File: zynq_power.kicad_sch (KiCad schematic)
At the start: 1 part, among them U2 XC7Z020-2CLG400I

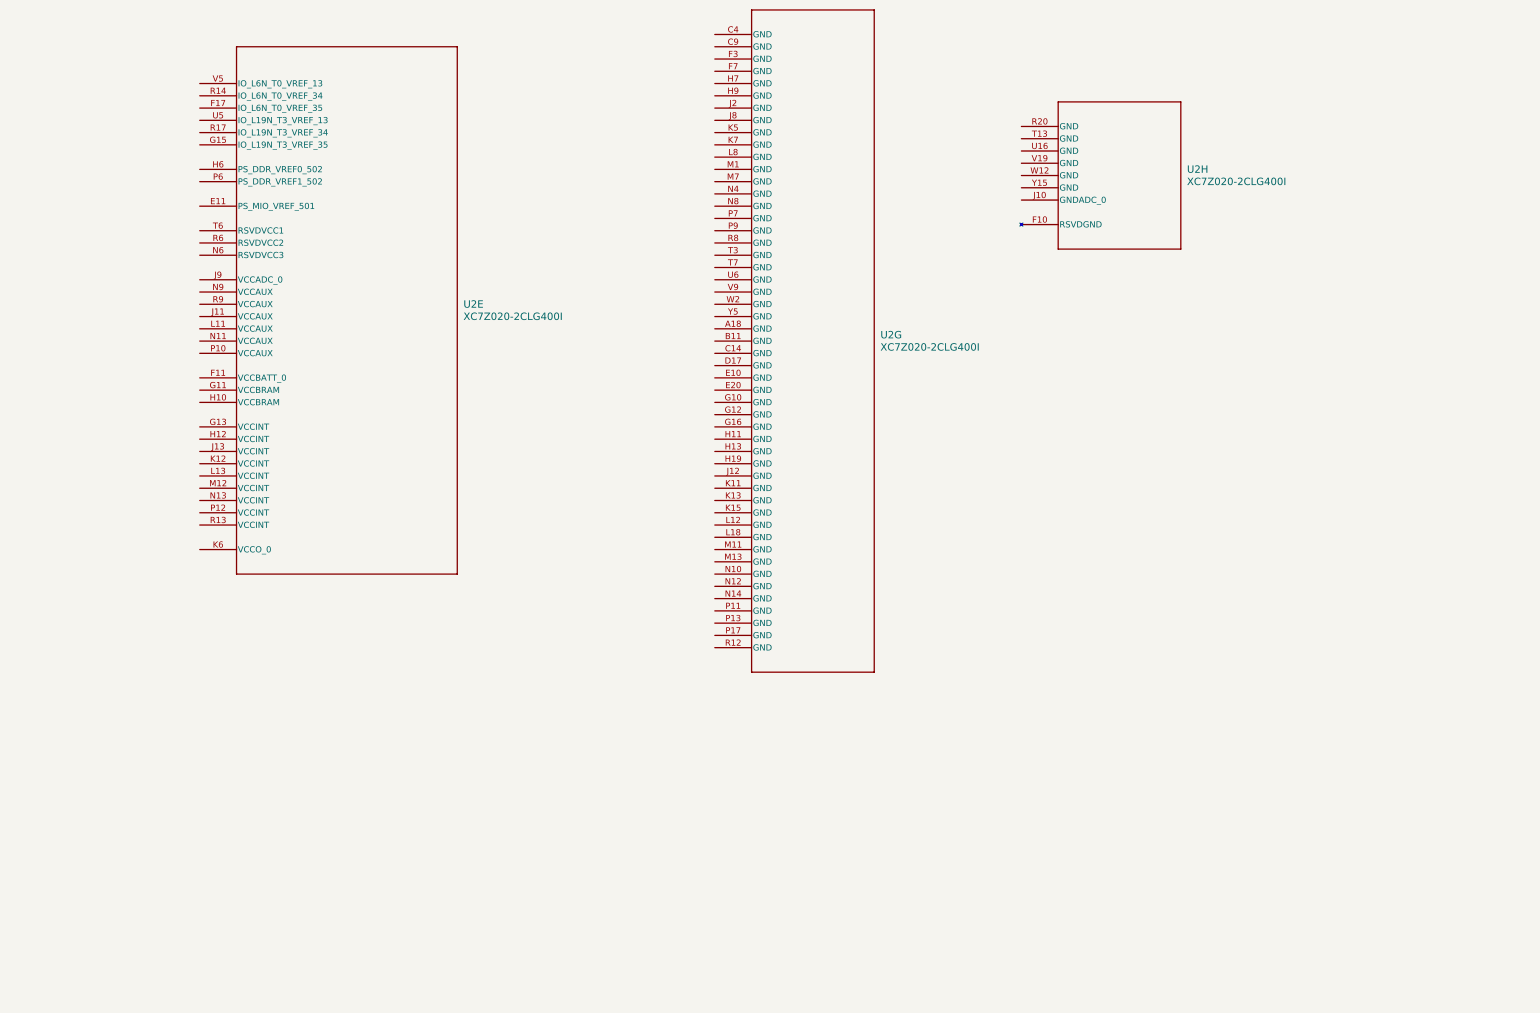
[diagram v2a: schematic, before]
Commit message: sch-updated
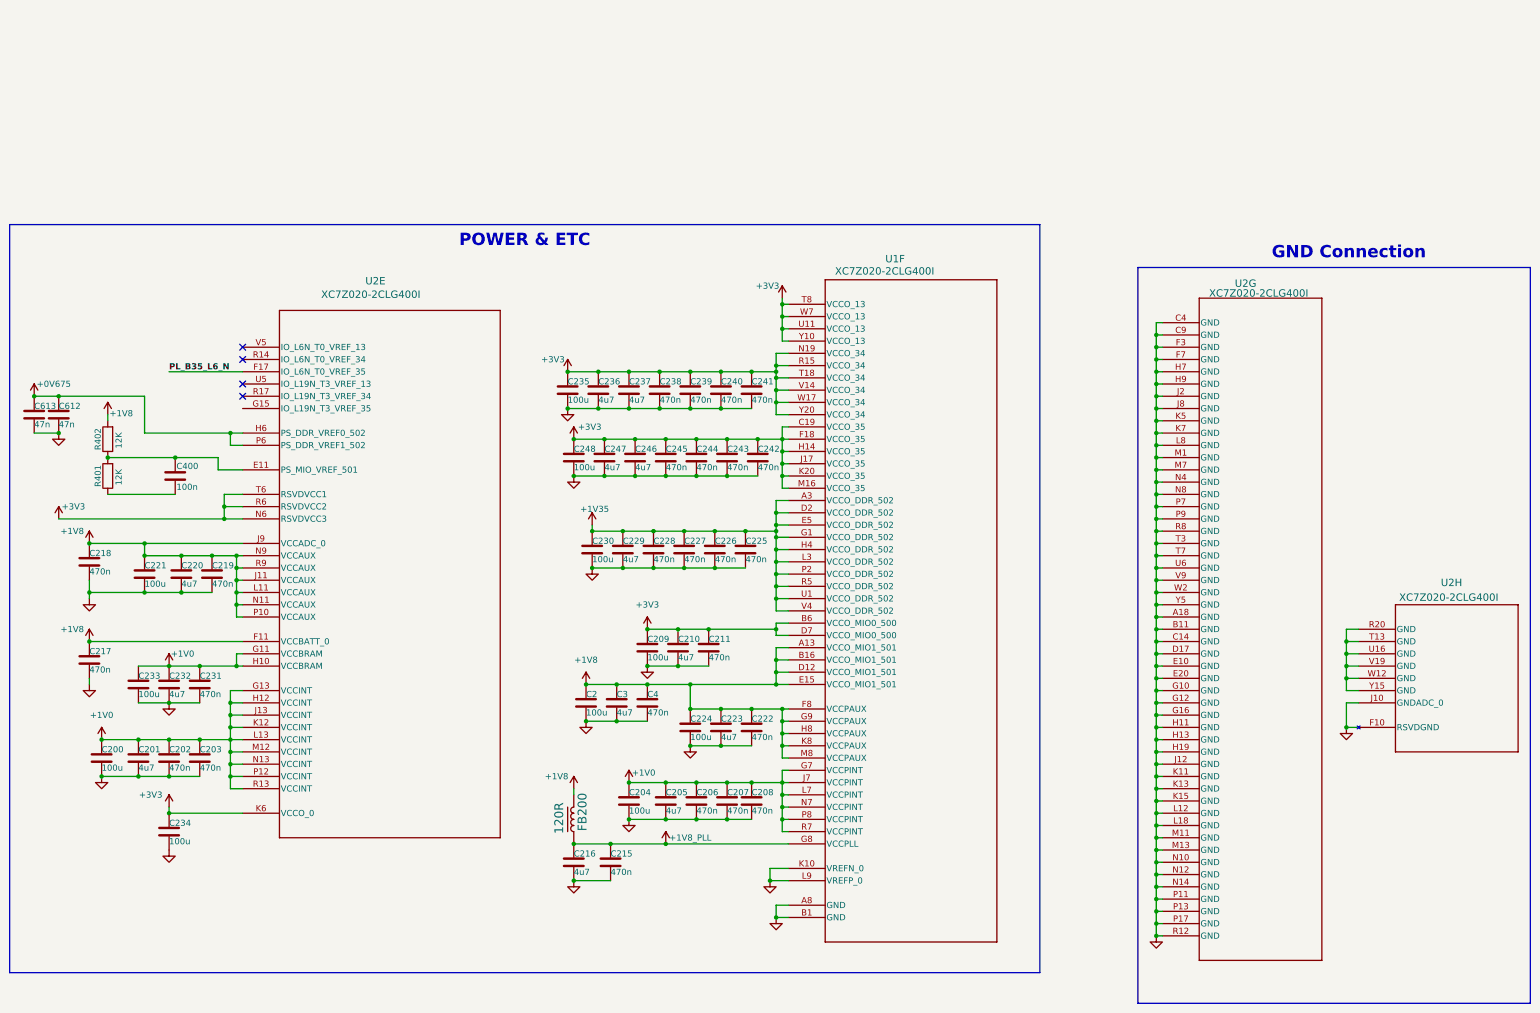
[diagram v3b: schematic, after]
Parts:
- added C2, C200, C204, C209, C221, C224, C230, C233, C234, C235, C248: 100u, Capacitor_SMD:C_1206_3216Metric, symbol Device:C
- added C201, C205, C210, C216, C220, C223, C229, C232, C236, C237, C246, C247, C3: 4u7, Capacitor_SMD:C_0402_1005Metric, symbol Device:C
- added C202, C203, C206, C207, C208, C211, C215, C217, C218, C219, C222, C225, C226, C227, C228, C231, C238, C239, C240, C241, C242, C243, C244, C245, C4: 470n, Capacitor_SMD:C_0402_1005Metric, symbol Device:C
- added C400: 100n, Capacitor_SMD:C_0402_1005Metric, symbol Device:C
- added C612, C613: 47n, Capacitor_SMD:C_0402_1005Metric, symbol Device:C
- added FB200: 120R, FB_0402, symbol Schematic-Lib-PhilsLab:FB_0402
- added R401, R402: 12K, Resistor_SMD:R_0402_1005Metric, symbol Device:R
- added U1: XC7Z020-2CLG400I, Package_BGA:Xilinx_CLG400, symbol 2024-11-30_12-42-37:XC7Z020-2CLG400I
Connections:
- net GND: now reaches U2.F10 (RSVDGND)
- net GND: now also U2.A18 (GND), U2.B11 (GND), U2.C14 (GND), U2.C4 (GND), U2.C9 (GND), U2.D17 (GND), U2.E10 (GND), U2.E20 (GND), U2.F3 (GND), U2.F7 (GND), U2.G10 (GND), U2.G12 (GND), U2.G16 (GND), U2.H11 (GND), U2.H13 (GND), U2.H19 (GND), U2.H7 (GND), U2.H9 (GND), U2.J10 (GNDADC_0), U2.J12 (GND), U2.J2 (GND), U2.J8 (GND), U2.K11 (GND), U2.K13 (GND), U2.K15 (GND), U2.K5 (GND), U2.K7 (GND), U2.L12 (GND), U2.L18 (GND), U2.L8 (GND), U2.M1 (GND), U2.M11 (GND), U2.M13 (GND), U2.M7 (GND), U2.N10 (GND), U2.N12 (GND), U2.N14 (GND), U2.N4 (GND), U2.N8 (GND), U2.P11 (GND), U2.P13 (GND), U2.P17 (GND), U2.P7 (GND), U2.P9 (GND), U2.R12 (GND), U2.R8 (GND), U2.T3 (GND), U2.T7 (GND), U2.U6 (GND), U2.V9 (GND), U2.W2 (GND), U2.Y5 (GND), C2.2, C200.2, C201.2, C202.2, C203.2, C204.2, C205.2, C206.2, C207.2, C208.2, C209.2, C210.2, C211.2, C215.2, C216.2, C217.2, C218.2, C219.2, C220.2, C221.2, C222.2, C223.2, C224.2, C225.2, C226.2, C227.2, C228.2, C229.2, C230.2, C231.2, C232.2, C233.2, C234.2, C235.2, C236.2, C237.2, C238.2, C239.2, C240.2, C241.2, C242.2, C243.2, C244.2, C245.2, C246.2, C247.2, C248.2, C3.2, C4.2, C612.2, C613.2, U1.A8 (GND), U1.B1 (GND), U1.K10 (VREFN_0), U1.L9 (VREFP_0)
- net at U2.R20 (GND): now also U2.T13 (GND), U2.U16 (GND), U2.V19 (GND), U2.W12 (GND), U2.Y15 (GND)
- net at U2.E11 (PS_MIO_VREF_501): now also C400.1, R401.2, R402.1
- net +1V8: now reaches U2.F11 (VCCBATT_0)
- net +1V8: now also U2.J11 (VCCAUX), U2.J9 (VCCADC_0), U2.L11 (VCCAUX), U2.N11 (VCCAUX), U2.N9 (VCCAUX), U2.P10 (VCCAUX), U2.R9 (VCCAUX), C2.1, C217.1, C218.1, C219.1, C220.1, C221.1, C222.1, C223.1, C224.1, C3.1, C4.1, FB200.2, R402.2, U1.A13 (VCCO_MIO1_501), U1.B16 (VCCO_MIO1_501), U1.D12 (VCCO_MIO1_501), U1.E15 (VCCO_MIO1_501), U1.F8 (VCCPAUX), U1.G9 (VCCPAUX), U1.H8 (VCCPAUX), U1.K8 (VCCPAUX), U1.M8 (VCCPAUX)
- net PL_B35_L6_N: now reaches U2.F17 (IO_L6N_T0_VREF_35)
- net +1V0: now reaches U2.G11 (VCCBRAM)
- net +1V0: now also U2.G13 (VCCINT), U2.H10 (VCCBRAM), U2.H12 (VCCINT), U2.J13 (VCCINT), U2.K12 (VCCINT), U2.L13 (VCCINT), U2.M12 (VCCINT), U2.N13 (VCCINT), U2.P12 (VCCINT), U2.R13 (VCCINT), C200.1, C201.1, C202.1, C203.1, C204.1, C205.1, C206.1, C207.1, C208.1, C231.1, C232.1, C233.1, U1.G7 (VCCPINT), U1.J7 (VCCPINT), U1.L7 (VCCPINT), U1.N7 (VCCPINT), U1.P8 (VCCPINT), U1.R7 (VCCPINT)
- net +0V675: now reaches U2.H6 (PS_DDR_VREF0_502)
- net +0V675: now also U2.P6 (PS_DDR_VREF1_502), C612.1, C613.1
- net +3V3: now reaches U2.K6 (VCCO_0)
- net +3V3: now also U2.N6 (RSVDVCC3), U2.R6 (RSVDVCC2), U2.T6 (RSVDVCC1), C209.1, C210.1, C211.1, C234.1, C235.1, C236.1, C237.1, C238.1, C239.1, C240.1, C241.1, C242.1, C243.1, C244.1, C245.1, C246.1, C247.1, C248.1, U1.B6 (VCCO_MIO0_500), U1.C19 (VCCO_35), U1.D7 (VCCO_MIO0_500), U1.F18 (VCCO_35), U1.H14 (VCCO_35), U1.J17 (VCCO_35), U1.K20 (VCCO_35), U1.M16 (VCCO_35), U1.N19 (VCCO_34), U1.R15 (VCCO_34), U1.T18 (VCCO_34), U1.T8 (VCCO_13), U1.U11 (VCCO_13), U1.V14 (VCCO_34), U1.W17 (VCCO_34), U1.W7 (VCCO_13), U1.Y10 (VCCO_13), U1.Y20 (VCCO_34)
- new net: C400.2, R401.1
- new net +1V35: C225.1, C226.1, C227.1, C228.1, C229.1, C230.1, U1.A3 (VCCO_DDR_502), U1.D2 (VCCO_DDR_502), U1.E5 (VCCO_DDR_502), U1.G1 (VCCO_DDR_502), U1.H4 (VCCO_DDR_502), U1.L3 (VCCO_DDR_502), U1.P2 (VCCO_DDR_502), U1.R5 (VCCO_DDR_502), U1.U1 (VCCO_DDR_502), U1.V4 (VCCO_DDR_502)
- new net +1V8_PLL: C215.1, C216.1, FB200.1, U1.G8 (VCCPLL)
- no-connect marks 0 -> 4
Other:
- note added: "GND Connection"
- note added: "POWER & ETC"
- moved on the sheet: U2E, U2G, U2H
